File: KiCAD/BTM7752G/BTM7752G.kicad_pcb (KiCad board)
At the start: 2 copper layers, 100 x 50 mm, 27 parts, among them CN1 CONN_RED_2_Power, CN2 CONN_WHITE_5, CN3 CONN_RED_2_Power, CN4 CONN_WHITE_5_RE, CN5 CONN_RED_2_Power, P1 CONN_4_KRP, SW1 SLIDE_SW, SW2 SLIDE_SW, U1 TA48M05F, U2 BTM7752G, U3 PSOC3_CY8C38_FAMILY_100, U4 pad_2mm_1.7mm, U5 pad_2mm_1.7mm

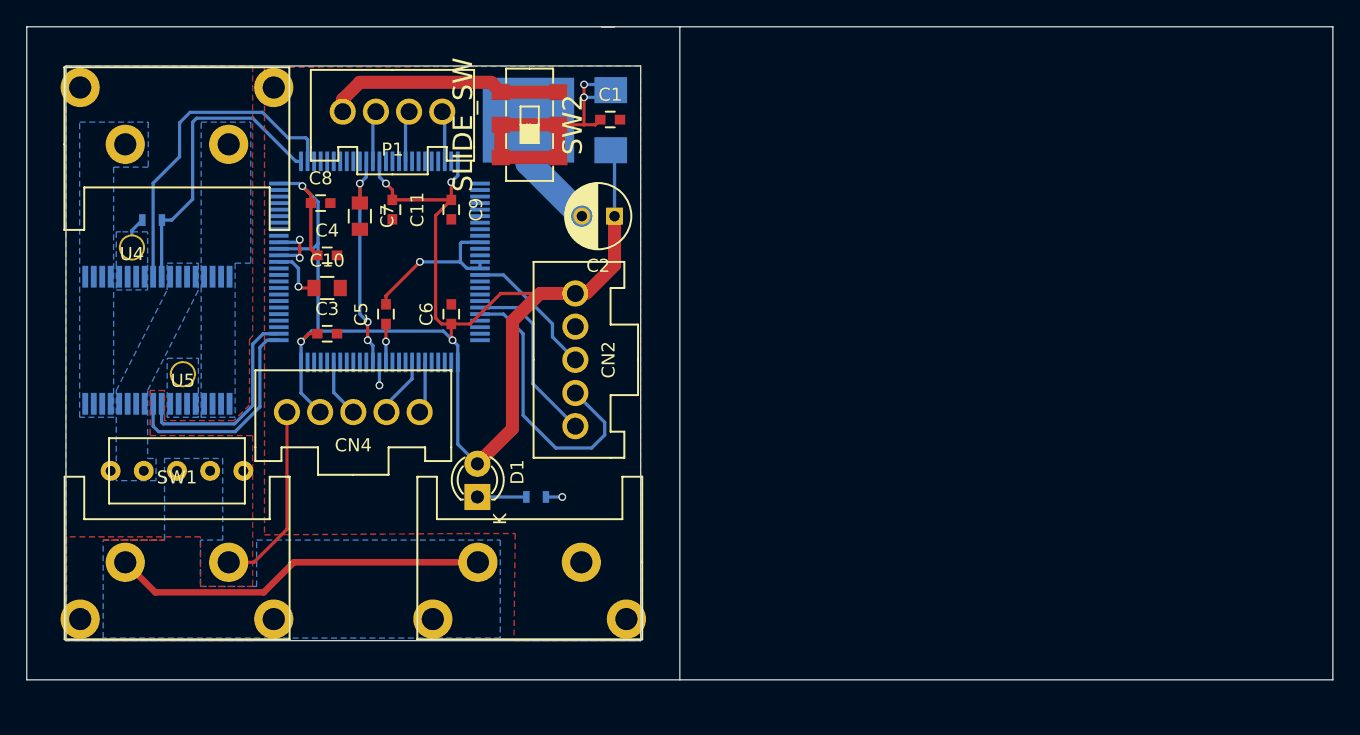
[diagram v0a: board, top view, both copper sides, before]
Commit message: update
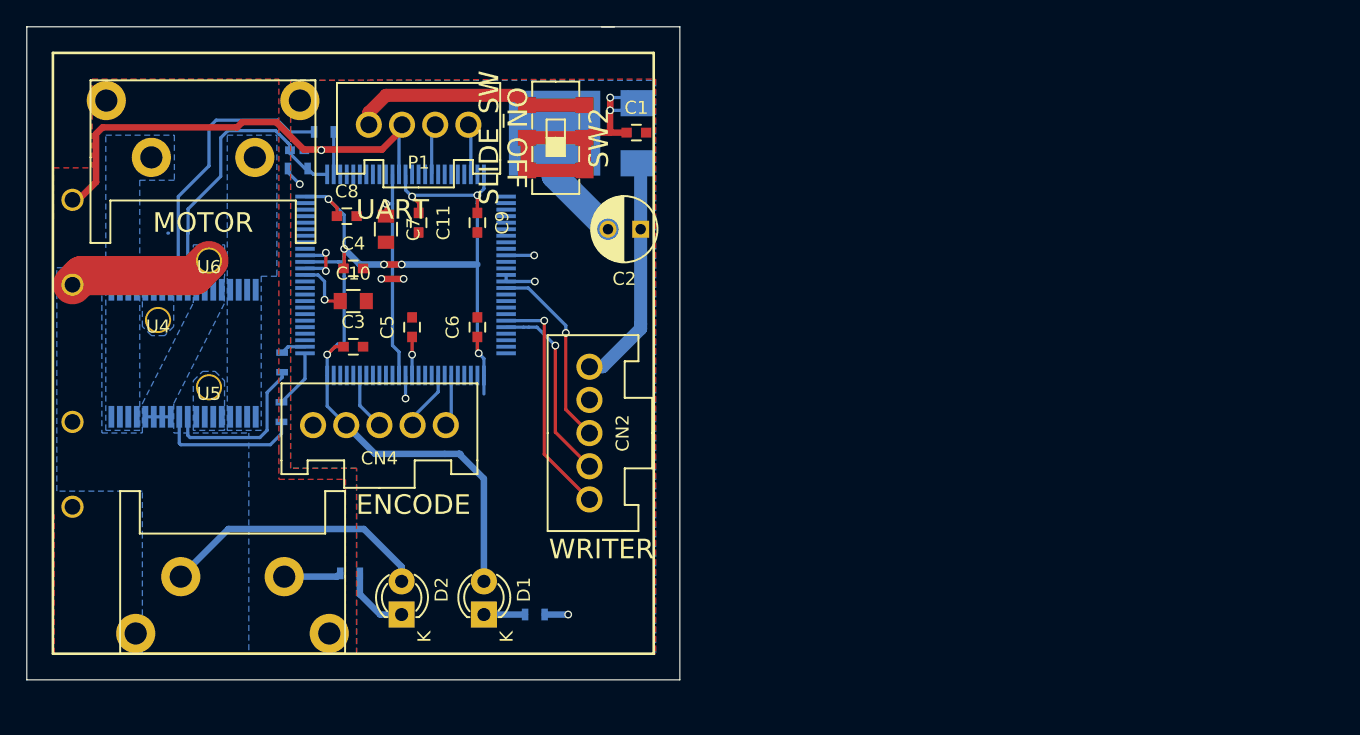
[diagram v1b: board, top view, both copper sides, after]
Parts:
- removed CN5: CONN_RED_2_Power, user_conn:CONN_RED_2P_STRAIGHT
- removed SW1: SLIDE_SW, user_SW:Toggle_Swith
- added C12: 1000u, user_drill:C_Radial_D18_L36_P7.5_Horizon5, B.Cu at (119.0, 83.0)
- added C13: 1000u, user_drill:C_Radial_D18_L36_P7.5_Horizon6, B.Cu at (119.0, 67.0)
- added D2: LED, LEDs:LED-3MM, F.Cu at (128.7, 95.0)
- added D3: D, user_drill:SOD-523_1, B.Cu at (120.7, 59.5)
- added R3: 10k, Resistors_SMD:R_0603, B.Cu at (124.8, 91.8)
- added R4: 4.7k, Resistors_SMD:R_0603, B.Cu at (119.5, 75.7)
- added R5: 4.7k, Resistors_SMD:R_0603, B.Cu at (119.5, 79.5)
- added R6: 4.7k, Resistors_SMD:R_0603, B.Cu at (122.8, 58.0)
- added U6: pad_2mm_1.7mm, user_drill:pad_2mm_1.7mm, F.Cu at (114.0, 67.9)
- CN1: value CONN_RED_2_Power -> DF22L-2P
- moved R2 11.8 mm to (120.8, 60.9)
- moved D1 9.01 mm to (135.0, 95.0)
- moved R1 9.00 mm to (138.9, 95.0)
- moved U4 5.90 mm to (110.0, 72.5)
- moved CN2 5.71 mm to (143.1, 81.1)
- moved CN1 4.39 mm to (115.8, 92.1)
- moved C1 2.24 mm to (146.7, 58.1)
- moved C10 2.24 mm to (125.0, 71.0)
- moved C11 2.24 mm to (130.0, 65.0)
- moved C2 2.24 mm to (147.0, 65.5)
- moved C3 2.24 mm to (125.0, 74.5)
- moved C4 2.24 mm to (125.0, 68.5)
- moved C5 2.24 mm to (129.5, 73.0)
- moved C6 2.24 mm to (134.5, 73.0)
- moved C7 2.24 mm to (127.5, 65.5)
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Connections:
- CN1 pad 1: Net-(CN1-Pad1) -> +24V
- U2 pad 10: IN1_2 -> Net-(R5-Pad1)
- U2 pad 27: INH1 -> Net-(R6-Pad2)
- U2 pad 9: IN1_1 -> Net-(R4-Pad1)
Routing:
- net +24V: track 0.00 -> 33.9 mm
- net Net-(CN1-Pad1): track 28.9 -> 0.00 mm
- net Net-(R6-Pad2): track 0.00 -> 22.1 mm
- net INH1: track 25.3 -> 3.25 mm
- net GND: track 50.3 -> 65.3 mm, vias 5 -> 8
- net IN1_1: track 16.0 -> 1.94 mm
- net IN1_2: track 17.8 -> 4.50 mm
- net Net-(R4-Pad1): track 0.00 -> 12.7 mm
- net Net-(R5-Pad1): track 0.00 -> 11.1 mm
- net +5V: track 117.4 -> 107.1 mm, vias 5 -> 8
- net Net-(CN2-Pad2): track 22.0 -> 14.7 mm, vias 0 -> 1
- net Net-(D2-Pad1): track 0.00 -> 5.44 mm
- net Net-(CN2-Pad1): track 13.7 -> 18.0 mm, vias 0 -> 1
- net Net-(CN2-Pad3): track 10.6 -> 14.7 mm, vias 0 -> 1
- net (no net): track 0.00 -> 1.75 mm, vias 0 -> 2
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- added copper zone on B.Cu, net +5V
- removed copper zone on B.Cu, net Net-(CN1-Pad1)
- removed copper zone on F.Cu, net Net-(CN1-Pad1)
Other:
- board size 100 x 50 mm -> 50 x 50 mm
- board text added: "ENCODE"
- board text added: "MOTOR"
- board text added: "ON OFF"
- board text added: "UART"
- board text added: "WRITER"
